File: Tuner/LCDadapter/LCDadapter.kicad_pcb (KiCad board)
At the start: 2 copper layers, 59 x 56 mm, 35 parts, among them J1 Conn_02x05_Odd_Even, J2 Conn_01x01, J3 Conn_01x01, J4 Conn_01x01, J5 Conn_01x01, Q1 2N3904, SW1 SW_Push, SW2 SW_Push, SW3 SW_Push, SW4 SW_Push, SW5 SW_Push, SW6 SW_Push, U1 PCF8574, U2 LCD-016N002L

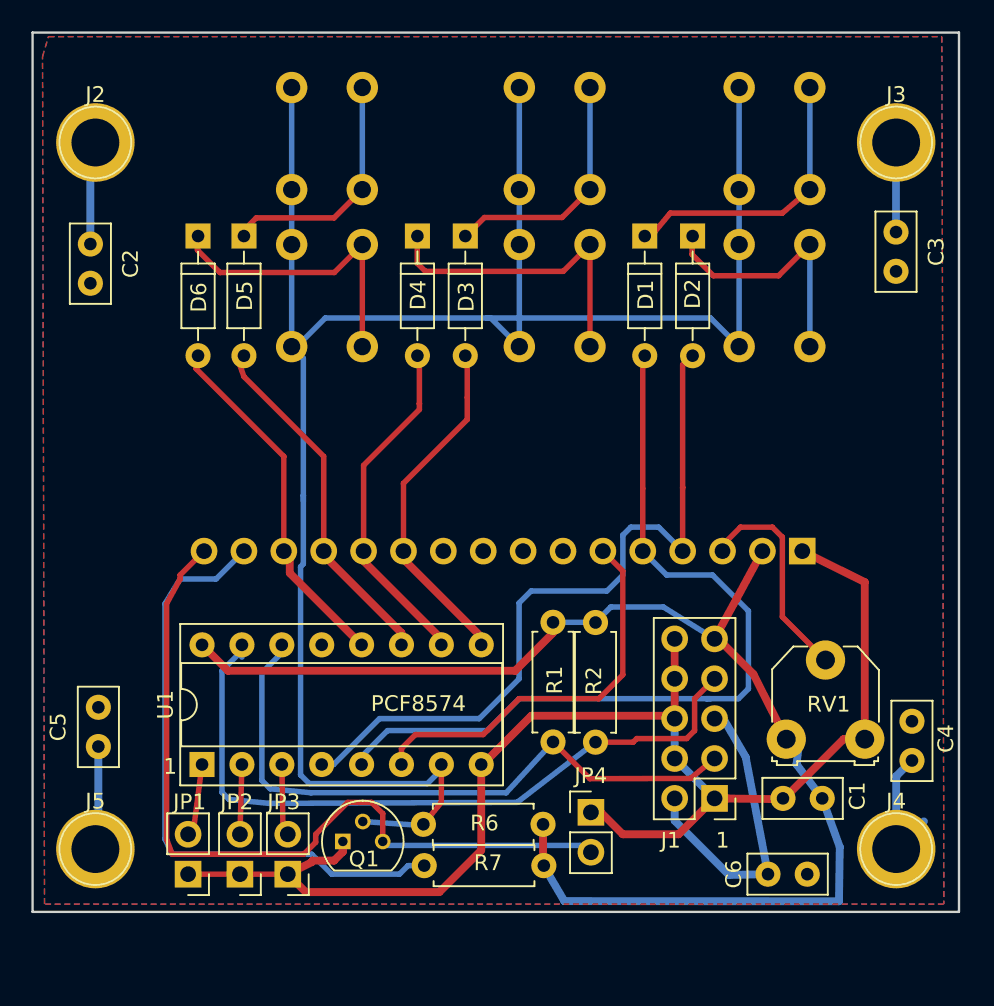
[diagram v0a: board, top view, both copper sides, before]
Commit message: LCDAdapter added dual polarity set I2C address
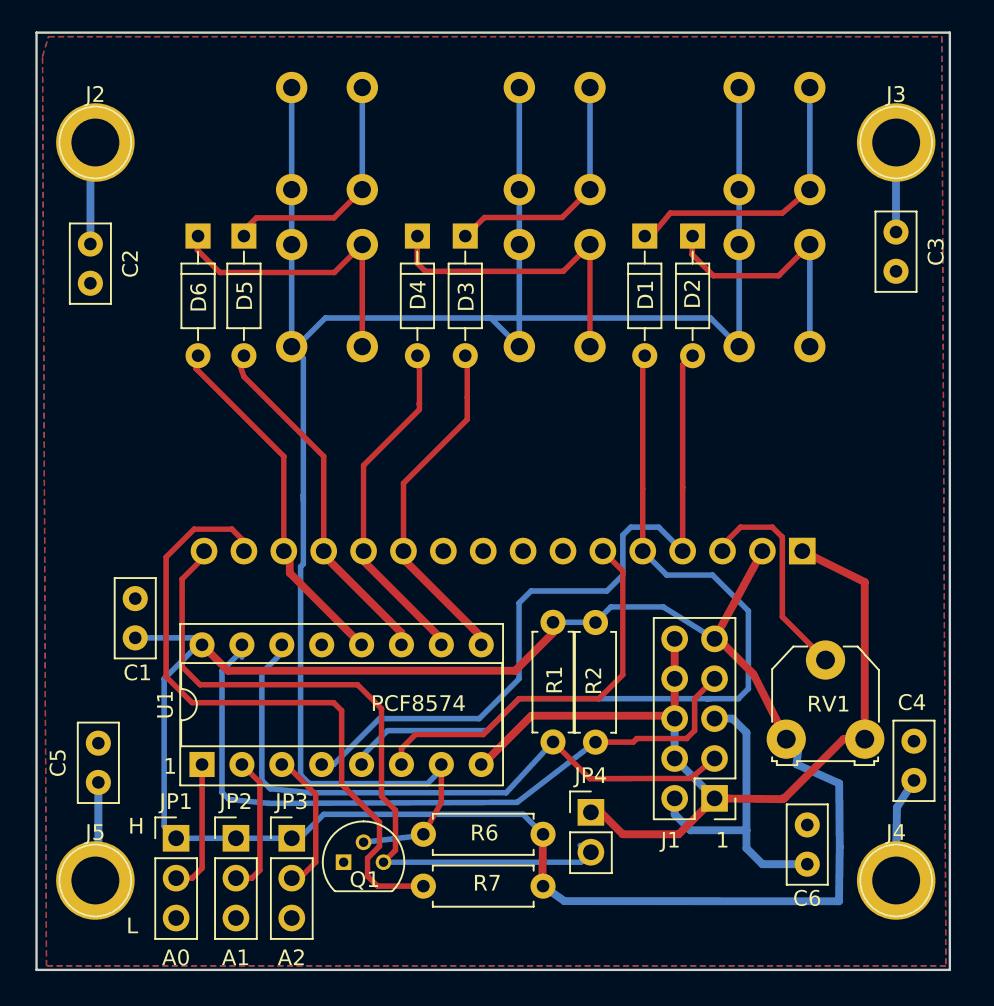
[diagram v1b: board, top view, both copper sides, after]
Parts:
- JP1, JP2, JP3: value Jumper -> Jumper_NC_Dual; footprint Pin_Headers:Pin_Header_Straight_1x02_Pitch2.54mm -> Pin_Headers:Pin_Header_Straight_1x03_Pitch2.54mm
- moved C1 44.9 mm to (117.5, 70.5), turned to 90 degrees
- moved C6 2.58 mm to (160.3, 85.0), turned to 90 degrees
- moved JP1 2.41 mm to (120.1, 83.3), turned to 0 degrees
- moved JP2 2.30 mm to (124.0, 83.3), turned to 0 degrees
- moved JP3 2.30 mm to (127.5, 83.3), turned to 0 degrees
- moved C5 2.29 mm to (115.2, 79.8)
- moved J4 2.00 mm to (166.0, 86.0)
- moved J5 2.00 mm to (115.0, 86.0)
- moved Q1 1.32 mm to (130.8, 84.8)
- moved R7 1.31 mm to (143.5, 86.4)
- moved C4 1.28 mm to (167.1, 79.6)
- moved R6 0.64 mm to (143.5, 83.1)
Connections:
- JP1 pad 1: GND -> +5V
- JP2 pad 1: GND -> +5V
- JP3 pad 1: GND -> +5V
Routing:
- net +5V: track 85.9 -> 129.4 mm
- net GND: track 91.5 -> 61.2 mm
- net Net-(JP3-Pad2): track 4.57 -> 9.21 mm
- net Net-(JP2-Pad2): track 4.45 -> 8.94 mm
- net Net-(JP4-Pad2): track 50.8 -> 46.7 mm
- net Net-(JP1-Pad2): track 4.63 -> 8.52 mm
- net Net-(C4-Pad1): track 8.56 -> 4.68 mm
- net Net-(R7-Pad2): track 40.0 -> 42.5 mm
- net Net-(C5-Pad1): track 6.61 -> 4.32 mm
- net Net-(C6-Pad1): track 19.8 -> 20.6 mm
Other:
- board size 59 x 56 mm -> 58.2 x 59.7 mm
- board text added: "A0"
- board text added: "A1"
- board text added: "A2"
- board text added: "H"
- board text added: "L"
